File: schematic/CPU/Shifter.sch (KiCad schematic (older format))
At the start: 10 parts, among them U19 74LS157, U20 74LS157, U21 74LS157, U22 74LS157, U23 74LS157, U24 74LS157, U25 74LS157, U26 74LS157, U27 74LS157, U28 74LS157

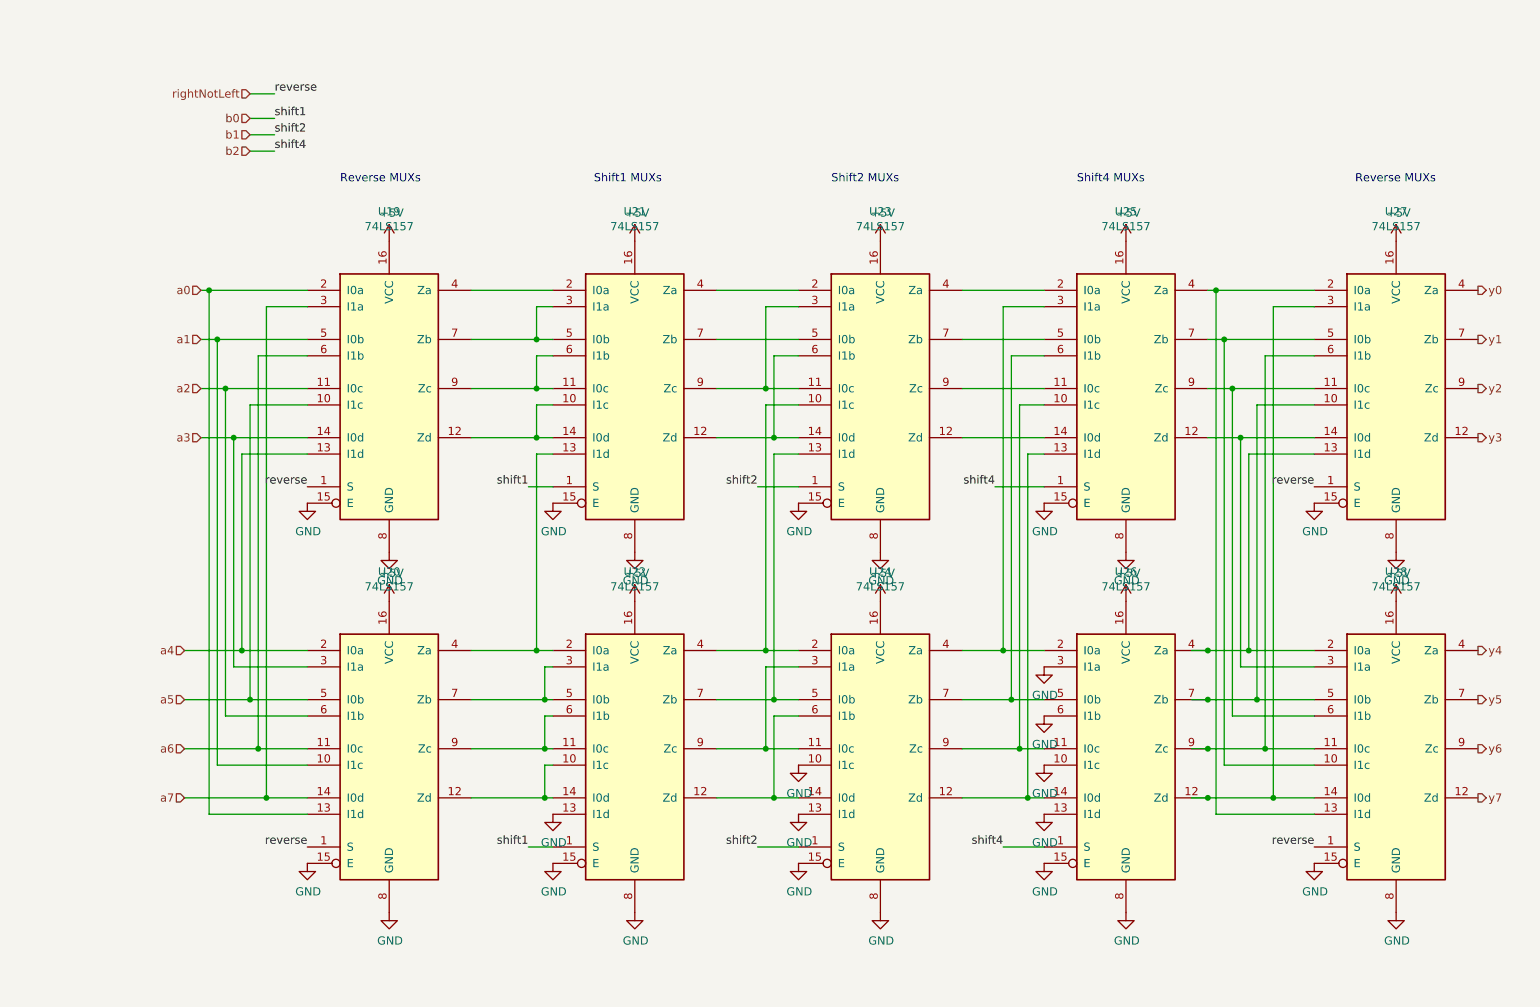
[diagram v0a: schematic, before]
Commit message: schematic finished
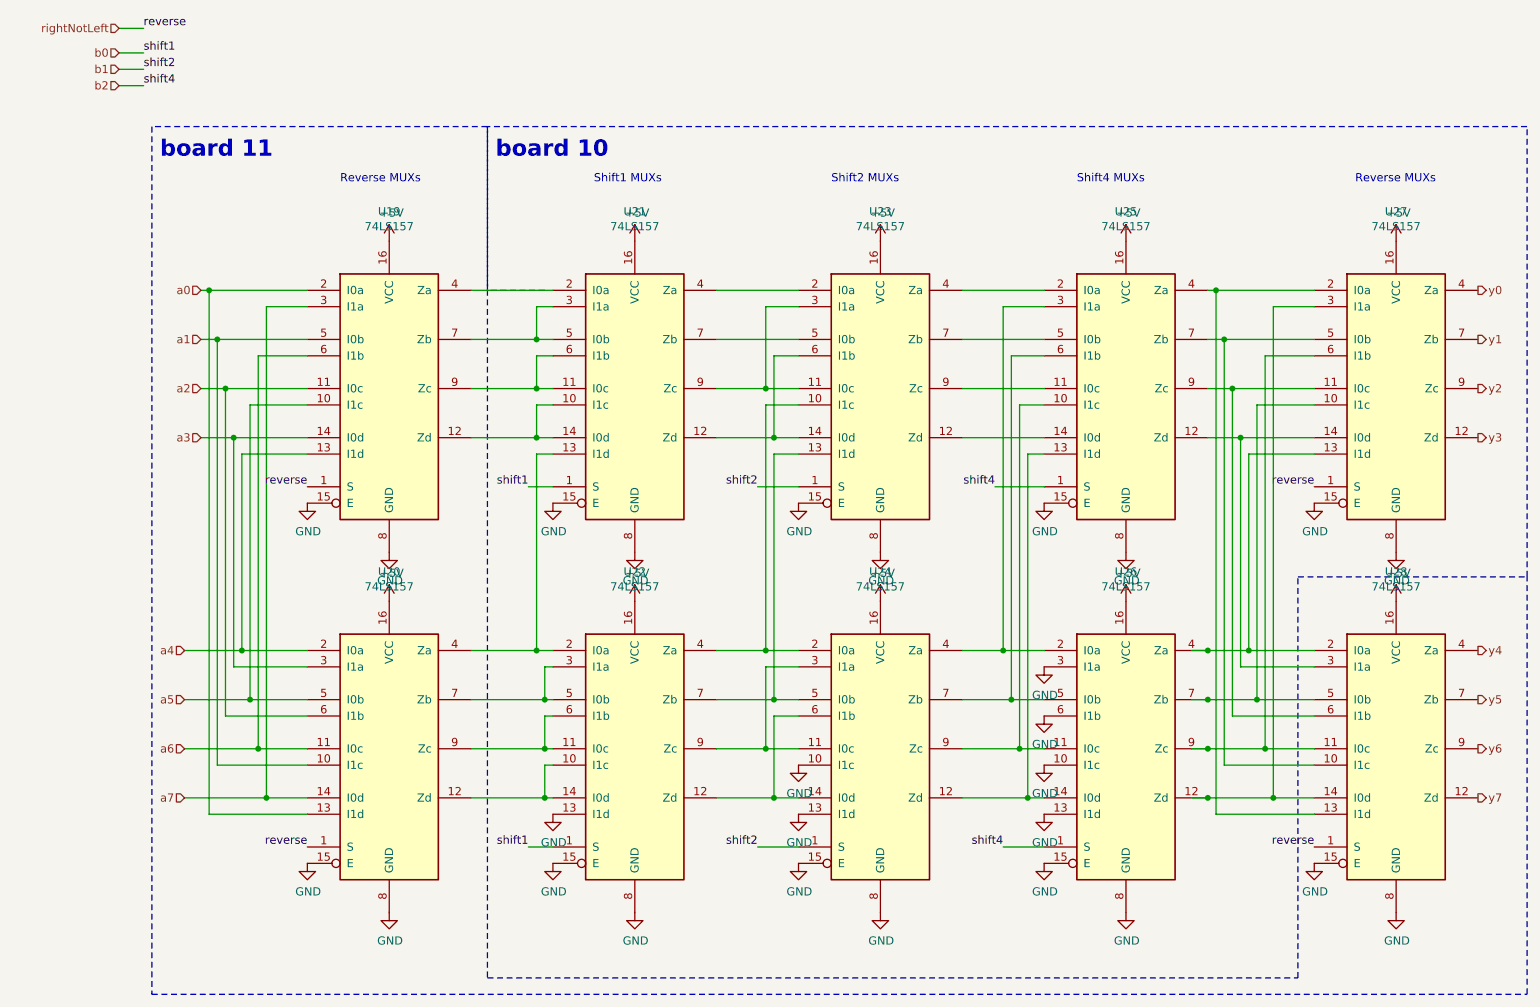
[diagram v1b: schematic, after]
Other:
- note added: "board 10"
- note added: "board 11\n"
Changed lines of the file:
@@
 Wire Wire Line
 	1900 5300 2150 5300
-Text Label 1950 1000 0    50   ~ 0
+Text Label 1150 600  0    50   ~ 0
 reverse
 Wire Wire Line
-	1950 1000 1800 1000
-Text HLabel 1800 1000 0    50   Input ~ 0
+	1150 600  1000 600
+Text HLabel 1000 600  0    50   Input ~ 0
 rightNotLeft
 $Comp
@@
 Wire Wire Line
 	6400 4400 6650 4400
-Text HLabel 1800 1150 0    50   Input ~ 0
+Text HLabel 1000 750  0    50   Input ~ 0
 b0
-Text HLabel 1800 1250 0    50   Input ~ 0
+Text HLabel 1000 850  0    50   Input ~ 0
 b1
-Text HLabel 1800 1350 0    50   Input ~ 0
+Text HLabel 1000 950  0    50   Input ~ 0
 b2
-Text Label 1950 1150 0    50   ~ 0
+Text Label 1150 750  0    50   ~ 0
 shift1
-Text Label 1950 1250 0    50   ~ 0
+Text Label 1150 850  0    50   ~ 0
 shift2
-Text Label 1950 1350 0    50   ~ 0
+Text Label 1150 950  0    50   ~ 0
 shift4
 Wire Wire Line
-	1800 1150 1950 1150
-Wire Wire Line
-	1800 1250 1950 1250
-Wire Wire Line
-	1950 1350 1800 1350
+	1000 750  1150 750
+Wire Wire Line
+	1000 850  1150 850
+Wire Wire Line
+	1150 950  1000 950
 Text Label 3500 3400 2    50   ~ 0
 shift1
@@
 	1    0    0    -1
 $EndComp
+Wire Notes Line width 12
+	3250 1200 3250 6400
+Wire Notes Line width 12
+	3250 6400 8200 6400
+Wire Notes Line width 12
+	8200 6400 8200 3950
+Wire Notes Line width 12
+	8200 3950 9600 3950
+Wire Notes Line width 12
+	9600 3950 9600 1200
+Wire Notes Line width 12
+	9600 1200 3250 1200
+Text Notes 3300 1400 0    100  ~ 20
+board 10
+Wire Notes Line
+	3600 2200 3250 2200
+Wire Notes Line
+	3250 2200 3250 1200
+Wire Notes Line width 12
+	3250 1200 1200 1200
+Wire Notes Line width 12
+	1200 1200 1200 6500
+Wire Notes Line width 12
+	1200 6500 9600 6500
+Wire Notes Line width 12
+	9600 6500 9600 3950
+Text Notes 1250 1400 0    100  ~ 20
+board 11\n
 $EndSCHEMATC
